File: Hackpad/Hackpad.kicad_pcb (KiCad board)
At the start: 2 copper layers, 45.2 x 69.1 mm, 7 parts, among them SW1 SW_Push, SW2 SW_Push, SW3 SW_Push, SW4 SW_Push, U1 XIAO-RP2040-DIP

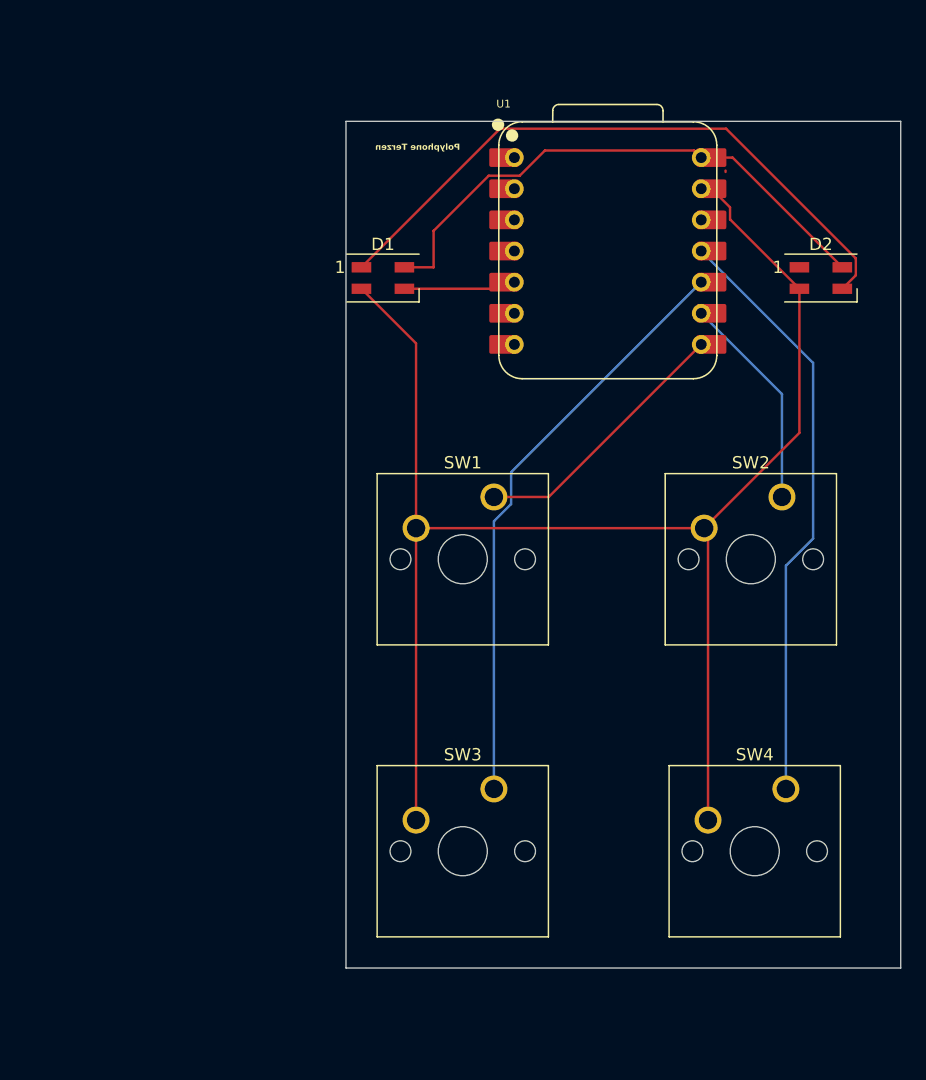
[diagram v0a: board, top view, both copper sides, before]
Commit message: updated pcb
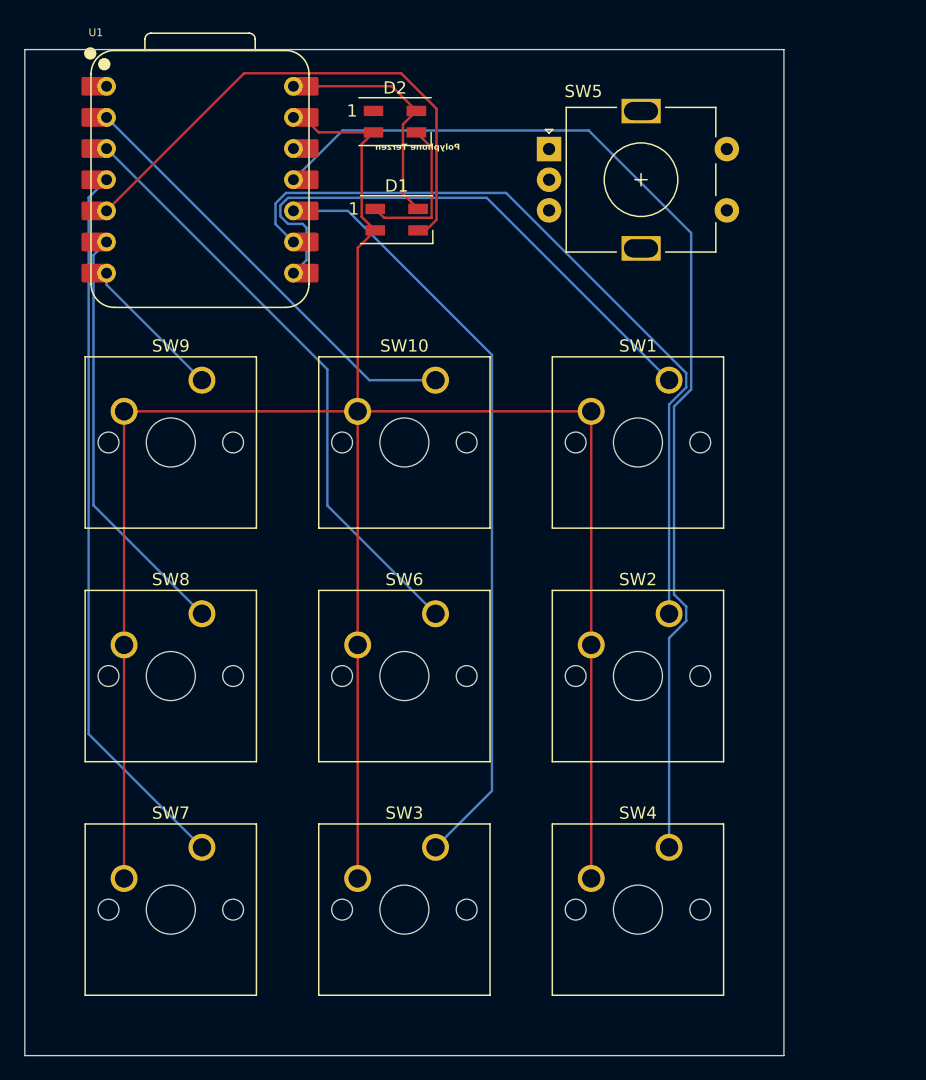
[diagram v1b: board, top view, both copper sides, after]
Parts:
- added SW10: SW_Push, Button_Switch_Keyboard:SW_Cherry_MX_1.00u_PCB, F.Cu at (81.1, 68.7)
- added SW5: RotaryEncoder, Rotary_Encoder:RotaryEncoder_Alps_EC11E-Switch_Vertical_H20mm, F.Cu at (90.4, 49.9)
- added SW6: SW_Push, Button_Switch_Keyboard:SW_Cherry_MX_1.00u_PCB, F.Cu at (81.1, 87.8)
- added SW7: SW_Push, Button_Switch_Keyboard:SW_Cherry_MX_1.00u_PCB, F.Cu at (62.1, 106.8)
- added SW8: SW_Push, Button_Switch_Keyboard:SW_Cherry_MX_1.00u_PCB, F.Cu at (62.1, 87.8)
- added SW9: SW_Push, Button_Switch_Keyboard:SW_Cherry_MX_1.00u_PCB, F.Cu at (62.1, 68.7)
- moved D2 37.0 mm to (77.8, 47.7)
- moved U1 33.8 mm to (61.9, 52.4)
- moved SW1 17.2 mm to (100.2, 68.7)
- moved SW2 13.2 mm to (100.2, 87.8)
- moved SW4 10.6 mm to (100.2, 106.8)
- moved SW3 6.74 mm to (81.1, 106.8)
- moved D1 4.89 mm to (78.0, 55.6)
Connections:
- U1 pad 2: unconnected-(U1-GPIO27/ADC1/A1-Pad2) -> Net-(U1-GPIO27/ADC1/A1)
- U1 pad 3: unconnected-(U1-GPIO28/ADC2/A2-Pad3) -> Net-(U1-GPIO28/ADC2/A2)
- U1 pad 4: unconnected-(U1-GPIO29/ADC3/A3-Pad4) -> Net-(U1-GPIO29/ADC3/A3)
- U1 pad 6: unconnected-(U1-GPIO7/SCL-Pad6) -> Net-(U1-GPIO7/SCL)
- U1 pad 7: unconnected-(U1-GPIO0/TX-Pad7) -> Net-(U1-GPIO0/TX)
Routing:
- net Net-(U1-GPIO29/ADC3/A3): track 0.00 -> 58.9 mm
- net GND: track 127.3 -> 182.8 mm
- net Net-(U1-GPIO28/ADC2/A2): track 0.00 -> 49.1 mm
- net Net-(U1-GPIO2/SCK): track 17.7 -> 63.9 mm
- net Net-(U1-GPIO3/MOSI): track 48.6 -> 89.3 mm
- net Net-(D1-DOUT): track 52.4 -> 12.4 mm
- net Net-(U1-GPIO27/ADC1/A1): track 0.00 -> 35.7 mm
- net Net-(D1-DIN): track 9.19 -> 43.7 mm
- net Net-(U1-GPIO7/SCL): track 0.00 -> 34.4 mm
- net +5V: track 45.3 -> 19.8 mm
- net Net-(U1-GPIO1/RX): track 22.1 -> 45.7 mm
- net Net-(U1-GPIO4/MISO): track 48.3 -> 63.1 mm
- net Net-(U1-GPIO0/TX): track 0.00 -> 12.0 mm
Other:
- board size 45.2 x 69.1 mm -> 61.9 x 82.1 mm

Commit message: finished pcb
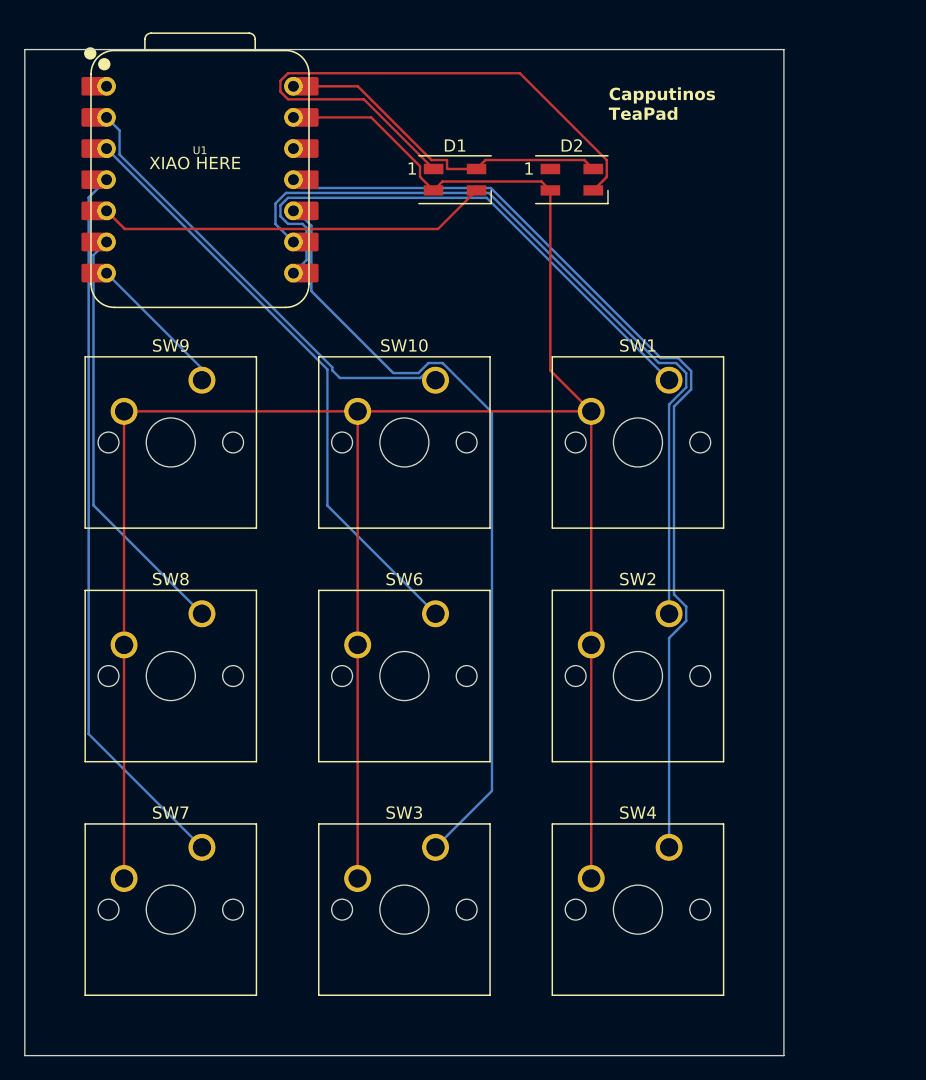
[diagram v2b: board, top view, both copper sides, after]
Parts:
- removed SW5: RotaryEncoder, Rotary_Encoder:RotaryEncoder_Alps_EC11E-Switch_Vertical_H20mm
- moved D2 15.2 mm to (92.2, 52.4)
- moved D1 5.77 mm to (82.7, 52.4)
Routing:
- net Net-(D1-DOUT): track 12.4 -> 48.7 mm
- net GND: track 182.8 -> 196.3 mm
- net Net-(D1-DIN): track 43.7 -> 32.4 mm
- net Net-(U1-GPIO3/MOSI): track 89.3 -> 79.3 mm
- net +5V: track 19.8 -> 29.2 mm
- net Net-(U1-GPIO27/ADC1/A1): track 35.7 -> 37.4 mm
- net Net-(U1-GPIO4/MISO): track 63.1 -> 64.2 mm
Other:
- board text added: "Capputinos TeaPad"
- board text added: "XIAO HERE"
- board text removed: "Polyphone Terzen"
